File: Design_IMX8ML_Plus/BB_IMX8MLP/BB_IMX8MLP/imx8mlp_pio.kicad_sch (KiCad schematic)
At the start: 2 parts, among them J3 DF40C-100DP-0.4V_51_, J4 DF40C-100DP-0.4V_51_

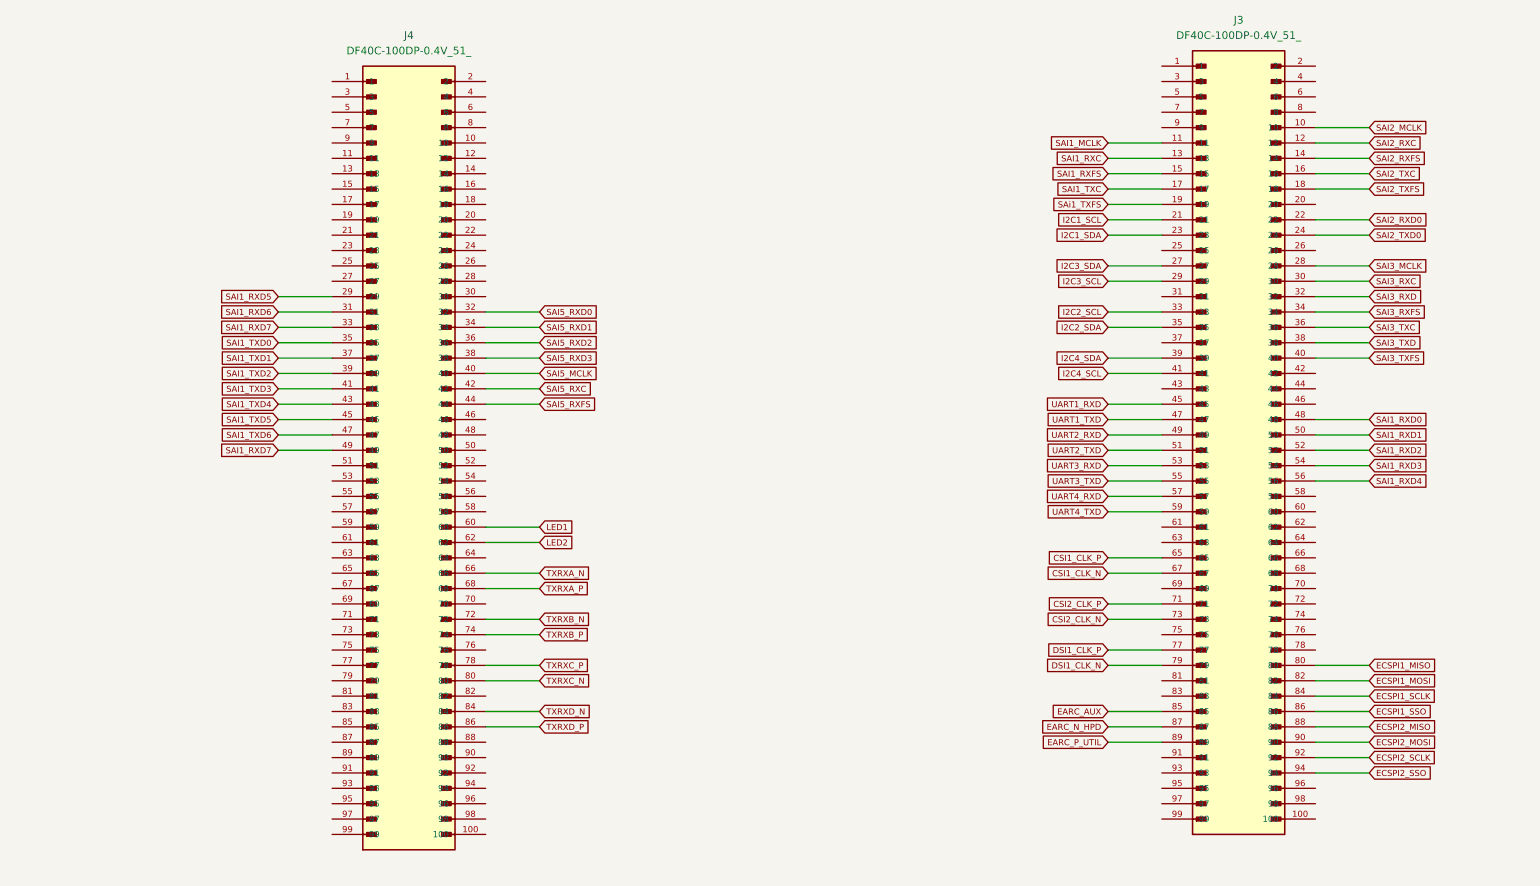
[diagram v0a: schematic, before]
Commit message: Add Base board IMxM8ML project
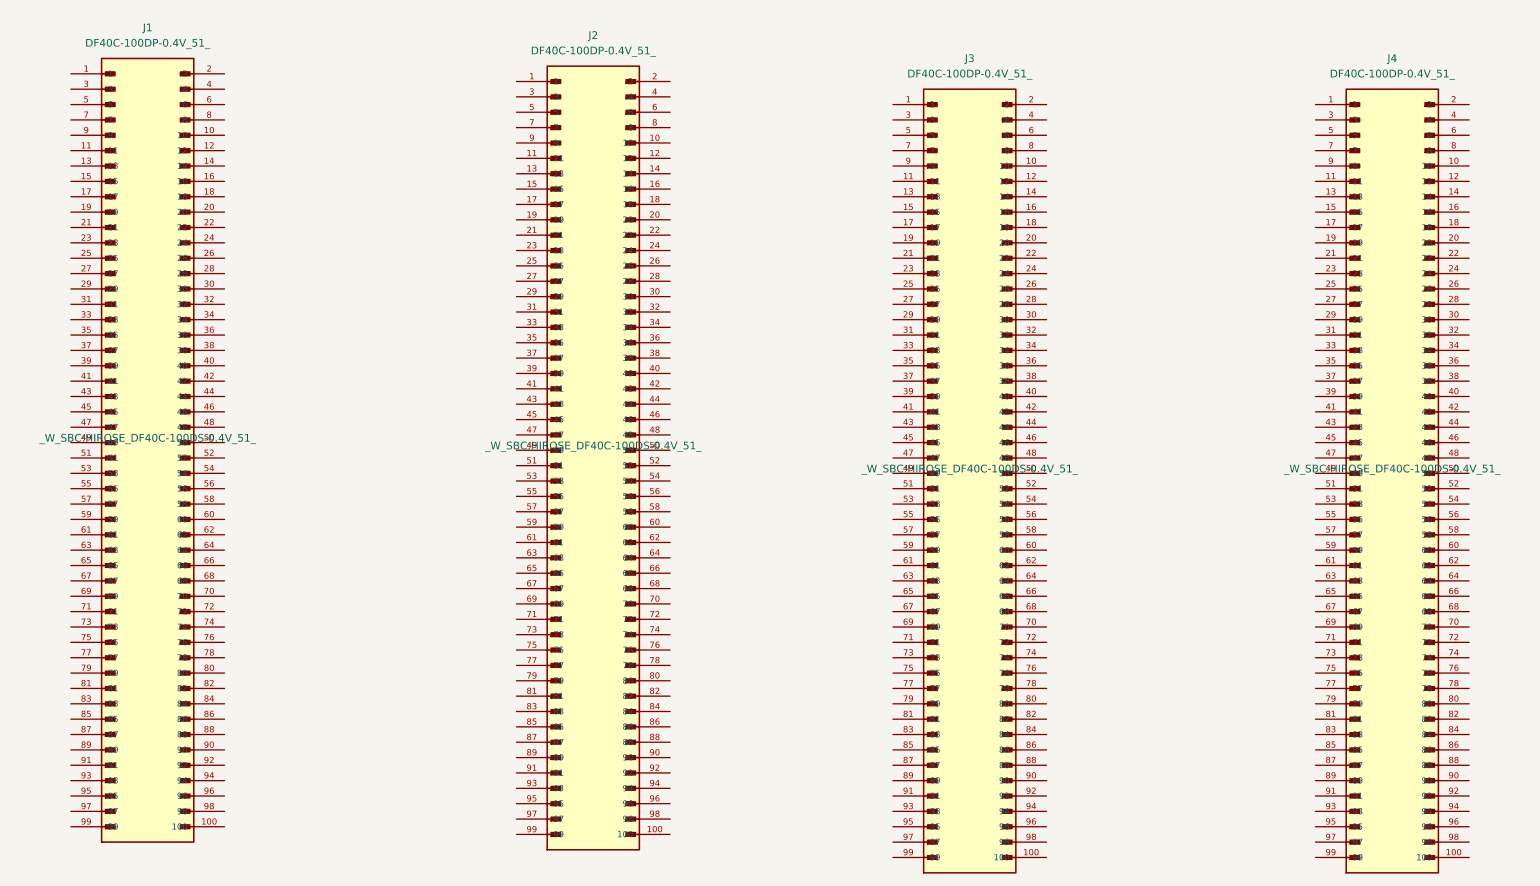
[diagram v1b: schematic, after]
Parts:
- added J1, J2: DF40C-100DP-0.4V_51_, _W_SBC:HIROSE_DF40C-100DS-0.4V_51_, symbol CONN_DF40C-100DS-0_4V51_HIR:DF40C-100DP-0.4V_51_
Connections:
- net CSI1_CLK_N: no longer names the net of J3.67
- net CSI1_CLK_P: no longer names the net of J3.65
- net CSI2_CLK_N: no longer names the net of J3.73
- net CSI2_CLK_P: no longer names the net of J3.71
- net DSI1_CLK_N: no longer names the net of J3.79
- net DSI1_CLK_P: no longer names the net of J3.77
- net EARC_AUX: no longer names the net of J3.85
- net EARC_N_HPD: no longer names the net of J3.87
- net EARC_P_UTIL: no longer names the net of J3.89
- net ECSPI1_MISO: no longer names the net of J3.80
- net ECSPI1_MOSI: no longer names the net of J3.82
- net ECSPI1_SCLK: no longer names the net of J3.84
- net ECSPI1_SSO: no longer names the net of J3.86
- net ECSPI2_MISO: no longer names the net of J3.88
- net ECSPI2_MOSI: no longer names the net of J3.90
- net ECSPI2_SCLK: no longer names the net of J3.92
- net ECSPI2_SSO: no longer names the net of J3.94
- net I2C1_SCL: no longer names the net of J3.21
- net I2C1_SDA: no longer names the net of J3.23
- net I2C2_SCL: no longer names the net of J3.33
- net I2C2_SDA: no longer names the net of J3.35
- net I2C3_SCL: no longer names the net of J3.29
- net I2C3_SDA: no longer names the net of J3.27
- net I2C4_SCL: no longer names the net of J3.41
- net I2C4_SDA: no longer names the net of J3.39
- net LED1: no longer names the net of J4.60
- net LED2: no longer names the net of J4.62
- net SAI1_MCLK: no longer names the net of J3.11
- net SAI1_RXC: no longer names the net of J3.13
- net SAI1_RXD0: no longer names the net of J3.48
- net SAI1_RXD1: no longer names the net of J3.50
- net SAI1_RXD2: no longer names the net of J3.52
- net SAI1_RXD3: no longer names the net of J3.54
- net SAI1_RXD4: no longer names the net of J3.56
- net SAI1_RXD5: no longer names the net of J4.29
- net SAI1_RXD6: no longer names the net of J4.31
- net SAI1_RXD7: no longer names the net of J4.33
- net SAI1_RXD7: no longer J4.49
- net SAI1_RXFS: no longer names the net of J3.15
- net SAI1_TXC: no longer names the net of J3.17
- net SAI1_TXD0: no longer names the net of J4.35
- net SAI1_TXD1: no longer names the net of J4.37
- net SAI1_TXD2: no longer names the net of J4.39
- net SAI1_TXD3: no longer names the net of J4.41
- net SAI1_TXD4: no longer names the net of J4.43
- net SAI1_TXD5: no longer names the net of J4.45
- net SAI1_TXD6: no longer names the net of J4.47
- net SAI2_MCLK: no longer names the net of J3.10
- net SAI2_RXC: no longer names the net of J3.12
- net SAI2_RXD0: no longer names the net of J3.22
- net SAI2_RXFS: no longer names the net of J3.14
- net SAI2_TXC: no longer names the net of J3.16
- net SAI2_TXD0: no longer names the net of J3.24
- net SAI2_TXFS: no longer names the net of J3.18
- net SAI3_MCLK: no longer names the net of J3.28
- net SAI3_RXC: no longer names the net of J3.30
- net SAI3_RXD: no longer names the net of J3.32
- net SAI3_RXFS: no longer names the net of J3.34
- net SAI3_TXC: no longer names the net of J3.36
- net SAI3_TXD: no longer names the net of J3.38
- net SAI3_TXFS: no longer names the net of J3.40
- net SAI5_MCLK: no longer names the net of J4.40
- net SAI5_RXC: no longer names the net of J4.42
- net SAI5_RXD0: no longer names the net of J4.32
- net SAI5_RXD1: no longer names the net of J4.34
- net SAI5_RXD2: no longer names the net of J4.36
- net SAI5_RXD3: no longer names the net of J4.38
- net SAI5_RXFS: no longer names the net of J4.44
- net SAi1_TXFS: no longer names the net of J3.19
- net TXRXA_N: no longer names the net of J4.66
- net TXRXA_P: no longer names the net of J4.68
- net TXRXB_N: no longer names the net of J4.72
- net TXRXB_P: no longer names the net of J4.74
- net TXRXC_N: no longer names the net of J4.80
- net TXRXC_P: no longer names the net of J4.78
- net TXRXD_N: no longer names the net of J4.84
- net TXRXD_P: no longer names the net of J4.86
- net UART1_RXD: no longer names the net of J3.45
- net UART1_TXD: no longer names the net of J3.47
- net UART2_RXD: no longer names the net of J3.49
- net UART2_TXD: no longer names the net of J3.51
- net UART3_RXD: no longer names the net of J3.53
- net UART3_TXD: no longer names the net of J3.55
- net UART4_RXD: no longer names the net of J3.57
- net UART4_TXD: no longer names the net of J3.59
